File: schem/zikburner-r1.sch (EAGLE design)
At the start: 16 parts, among them IC1 AT28C256, U1 ATMEGA644-20PU, U2 FT232RLSSOP, X2 USB-SMD-NS

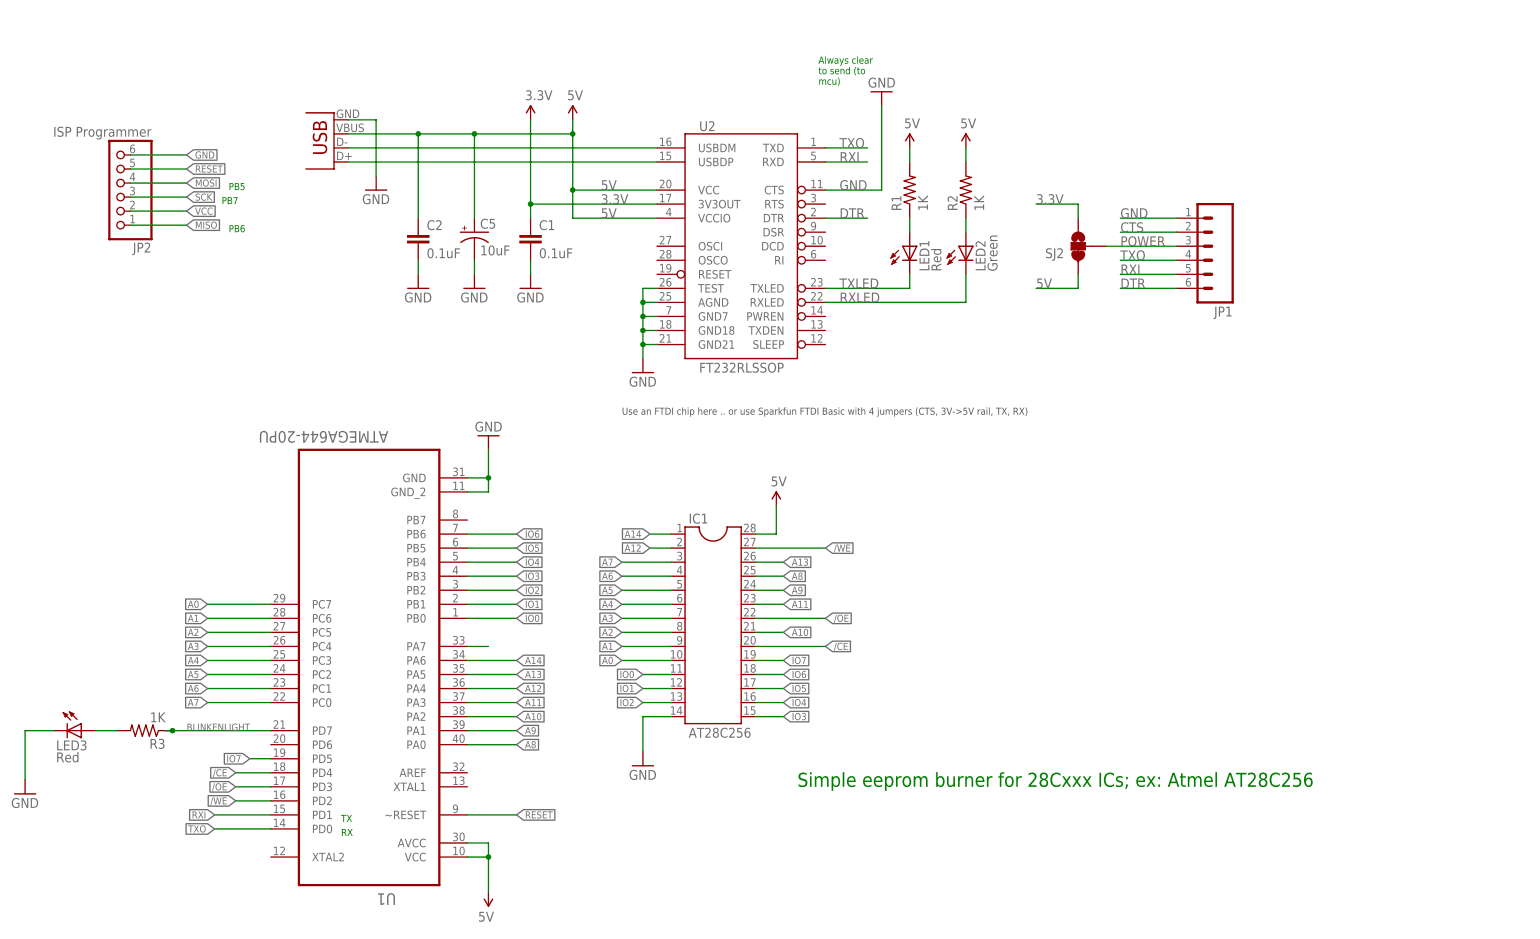
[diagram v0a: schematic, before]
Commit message: Fix to schematic
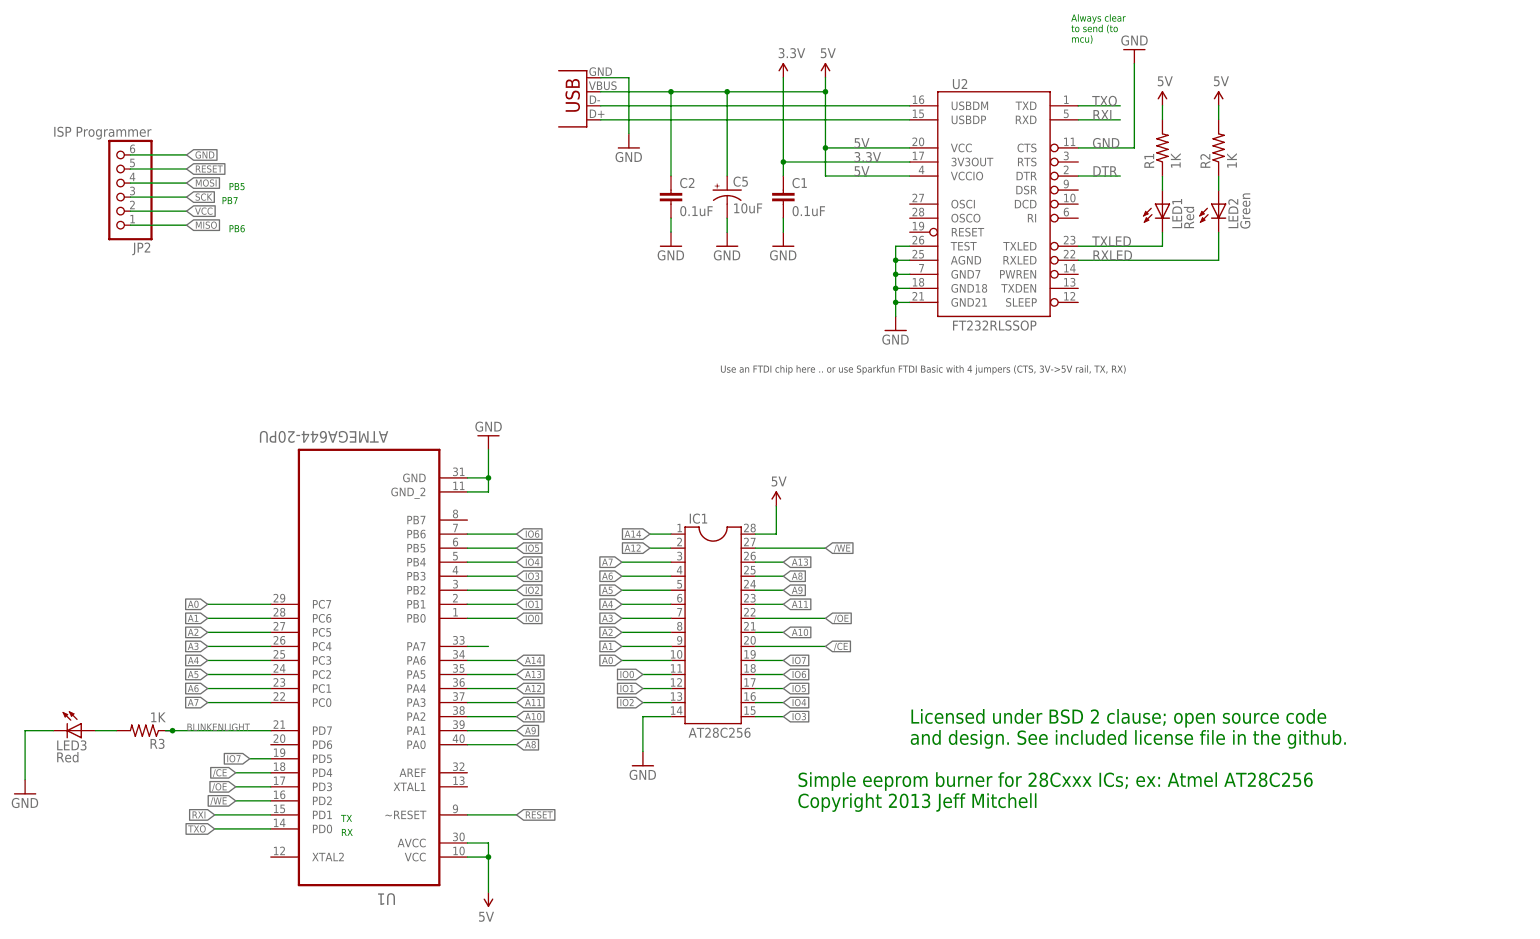
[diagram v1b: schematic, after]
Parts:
- removed JP1: (no value), SparkFun:M06SMD-FEMALE-V2
- removed SJ2: (no value), SparkFun:SOLDERJUMPER_2WAYS
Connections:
- removed net CTS: JP1.2
- removed net POWER: JP1.3, SJ2.2
- net 3.3V: no longer SJ2.3
- net 5V: no longer SJ2.1
- net DTR: no longer JP1.6
- net GND: no longer JP1.1
- net RXI: no longer JP1.5
- net TXO: no longer JP1.4
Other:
- note added: "Licensed under BSD 2 clause; open source code and design. See included license file in the github."
- note added: "Simple eeprom burner for 28Cxxx ICs; ex: Atmel AT28C256 Copyright 2013 Jeff Mitchell"
- note removed: "Simple eeprom burner for 28Cxxx ICs; ex: Atmel AT28C256"
- moved on the sheet: C1, C2, C5, LED1, LED2, R1, R2, U2
